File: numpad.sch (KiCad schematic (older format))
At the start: 60 parts, among them SW1 RESET, SW2 BOOT

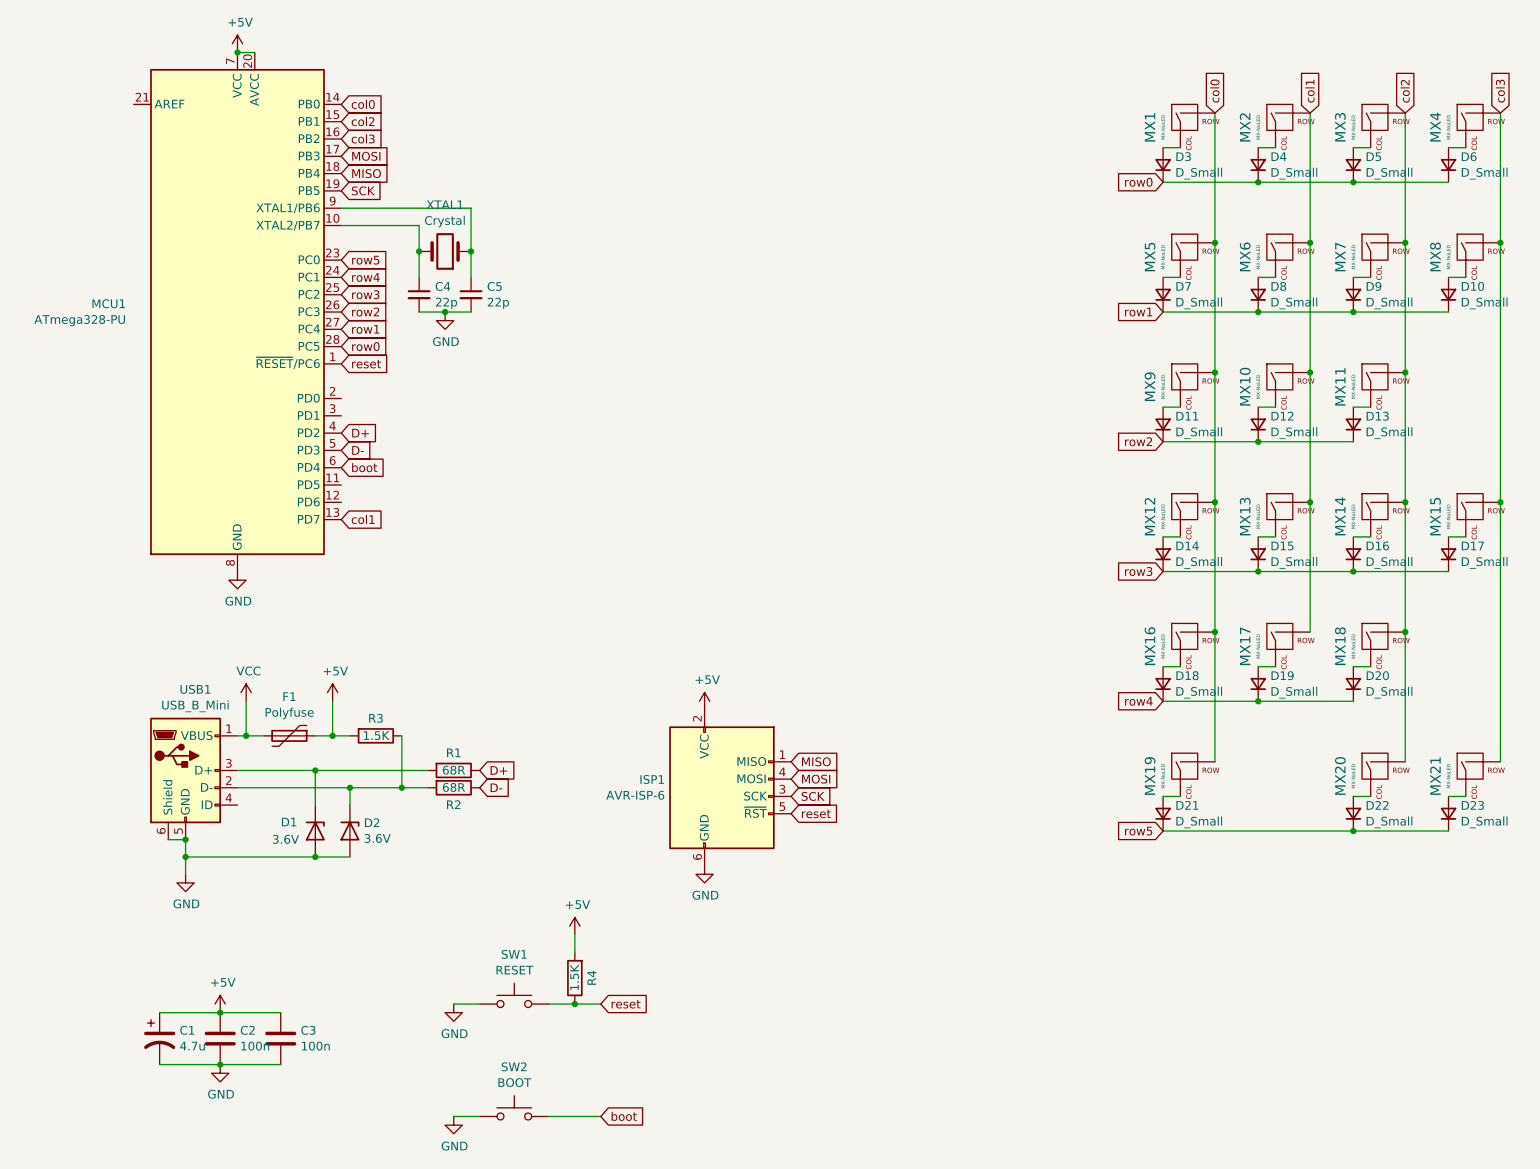
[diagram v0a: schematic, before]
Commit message: update
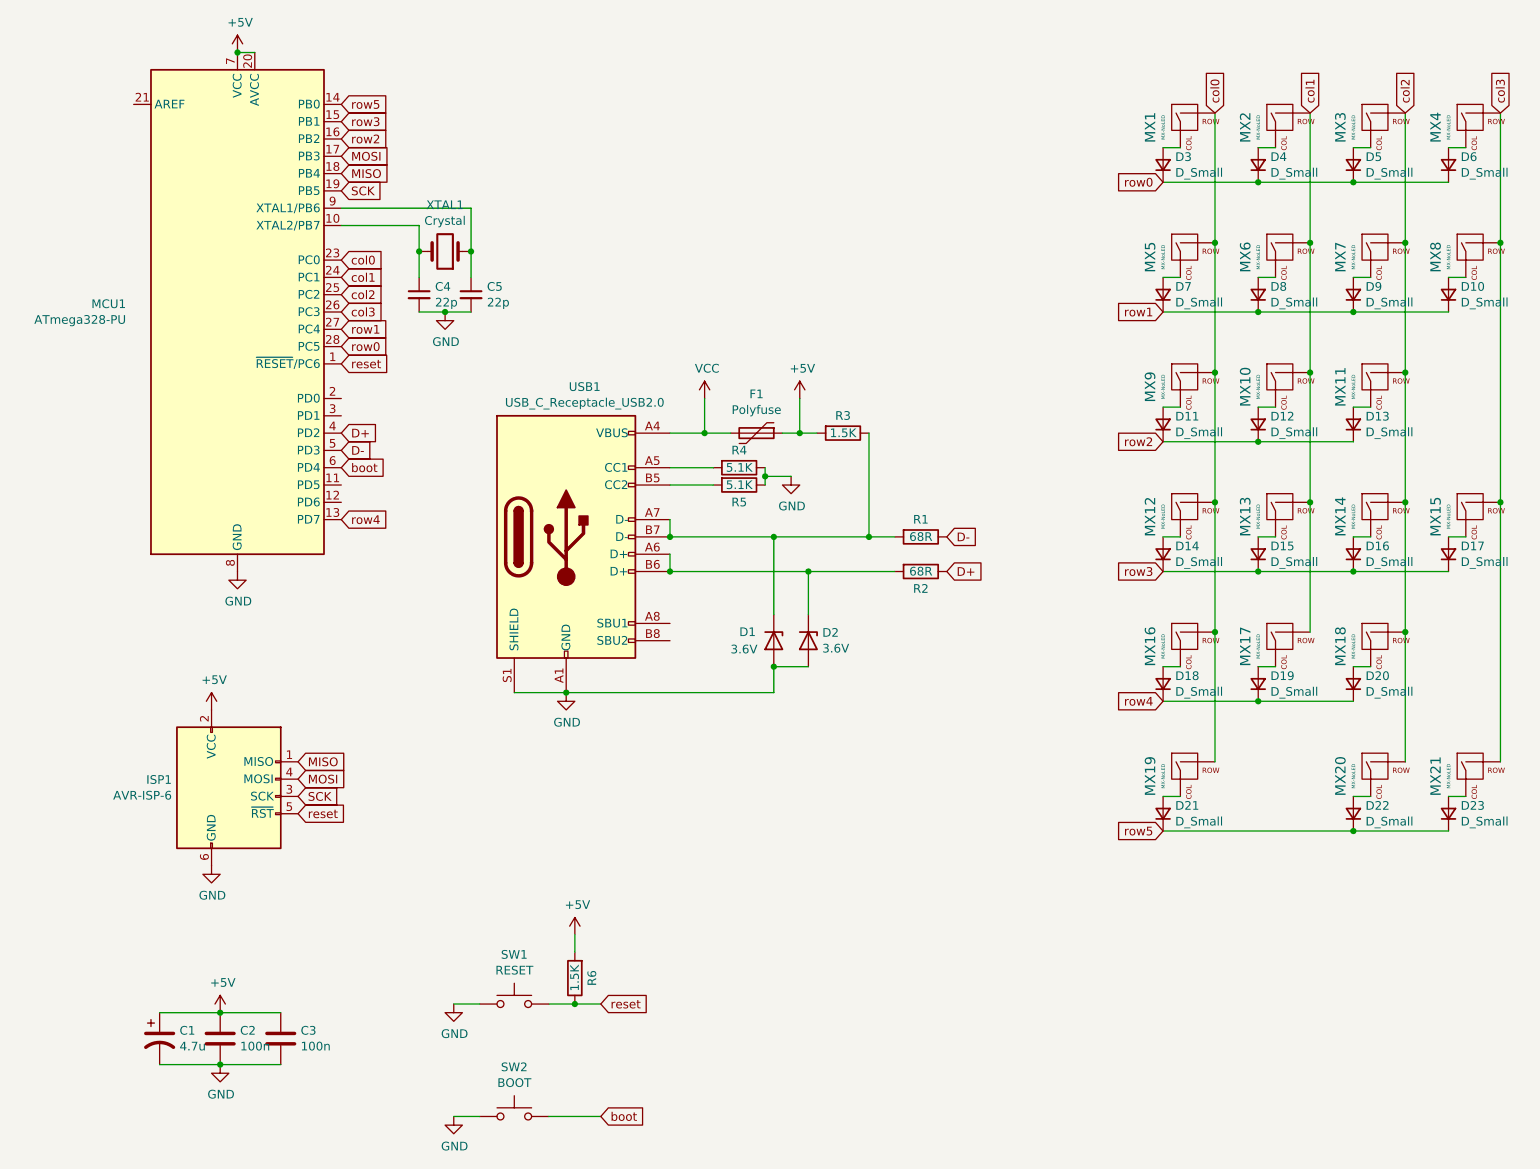
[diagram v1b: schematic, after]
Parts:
- removed USB1: USB_B_Mini, custom_parts:USB_Mini, symbol Connector:USB_B_Mini
- added R4, R5: 5.1K, Resistor_THT:R_Axial_DIN0204_L3.6mm_D1.6mm_P7.62mm_Horizontal, symbol Device:R
- added USB1: USB_C_Receptacle_USB2.0, custom_parts:USB_C_GCT_USB4085, symbol Connector:USB_C_Receptacle_USB2.0
- renumbered R4 to R6
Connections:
- net D+: now also R2.1; no longer R1.1
- net D-: now also R1.1; no longer R2.1
- net GND: now also R4.1, R5.1, USB1.A1 (GND), USB1.A12 (GND), USB1.B1 (GND), USB1.B12 (GND), USB1.S1 (SHIELD)
- net VCC: now also USB1.A4 (VBUS), USB1.A9 (VBUS), USB1.B4 (VBUS), USB1.B9 (VBUS)
- net col0: now also MCU1.23 (PC0); no longer MCU1.14 (PB0)
- net col1: now also MCU1.24 (PC1); no longer MCU1.13 (PD7)
- net col2: now also MCU1.25 (PC2); no longer MCU1.15 (PB1)
- net col3: now also MCU1.26 (PC3); no longer MCU1.16 (PB2)
- net row2: now also MCU1.16 (PB2); no longer MCU1.26 (PC3)
- net row3: now also MCU1.15 (PB1); no longer MCU1.25 (PC2)
- net row4: now also MCU1.13 (PD7); no longer MCU1.24 (PC1)
- net row5: now also MCU1.14 (PB0); no longer MCU1.23 (PC0)
- net at D2.1 (K), R2.2: now also USB1.A6 (D+), USB1.B6 (D+); no longer R3.1
- net at D1.1 (K), R1.2: now also R3.1, USB1.A7 (D-), USB1.B7 (D-)
- new net: R4.2, USB1.A5 (CC1)
- new net: R5.2, USB1.B5 (CC2)
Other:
- moved on the sheet: D1, D2, F1, ISP1, R1, R2, R3
